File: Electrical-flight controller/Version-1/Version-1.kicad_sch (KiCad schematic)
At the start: 19 parts, among them J1 USB_B_Micro, U1 ESP32-WROOM-32, U2 W25Q32JVZP, U4 CP2102N-Axx-xQFN28, Y1 Crystal_GND24

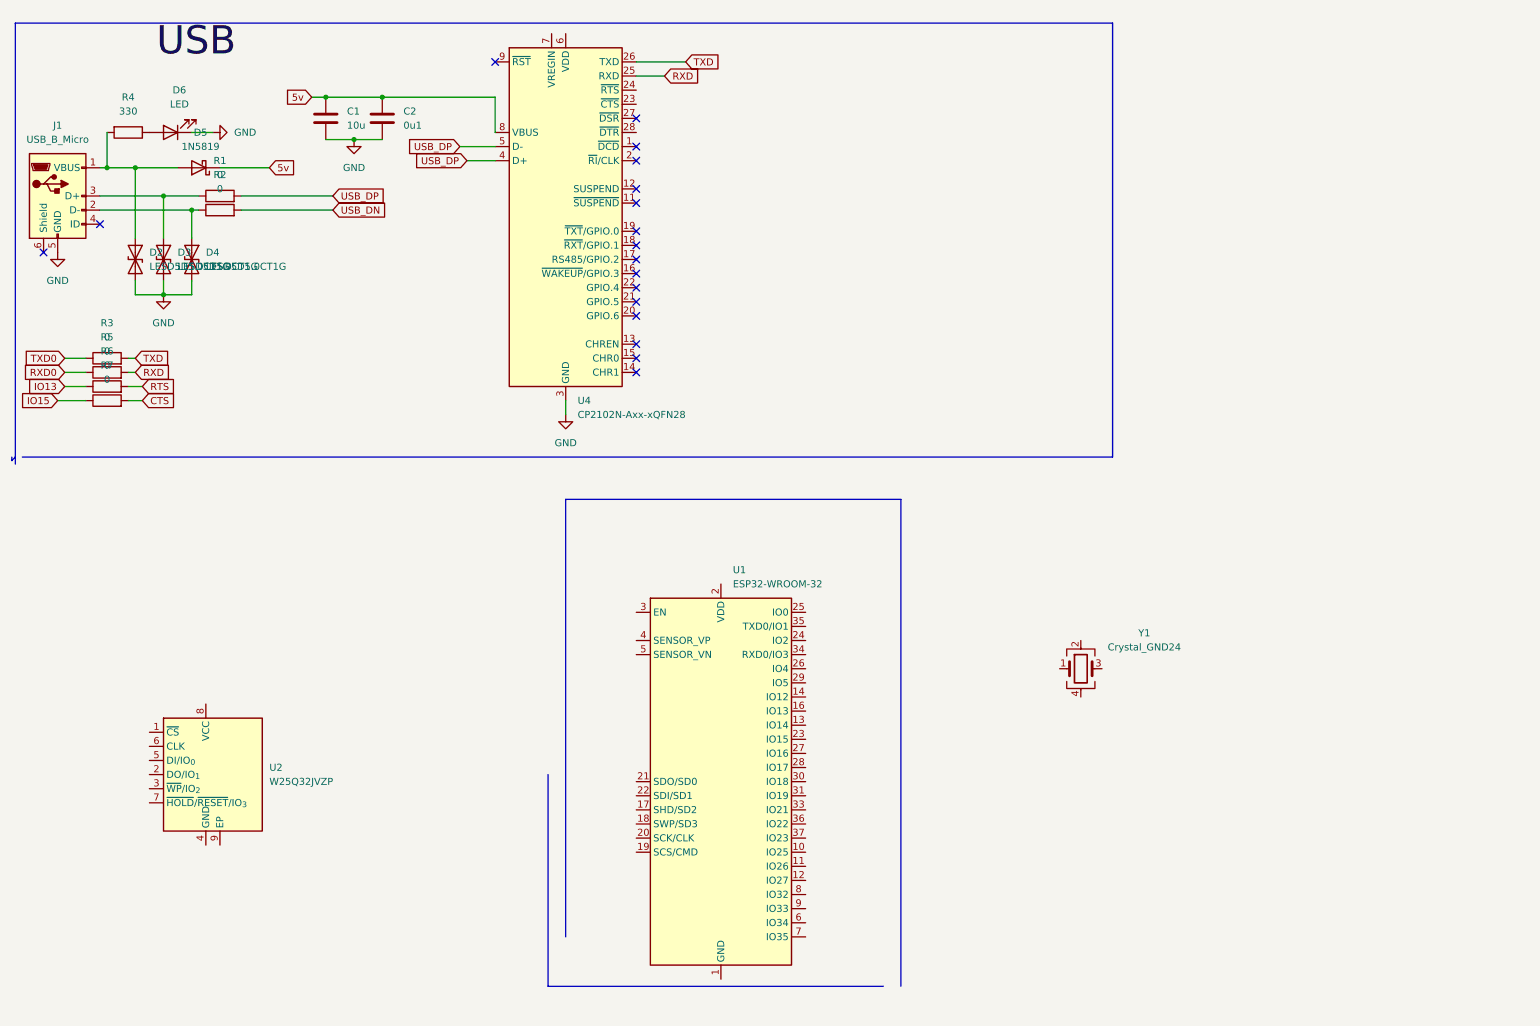
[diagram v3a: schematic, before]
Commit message: Pwoer supply
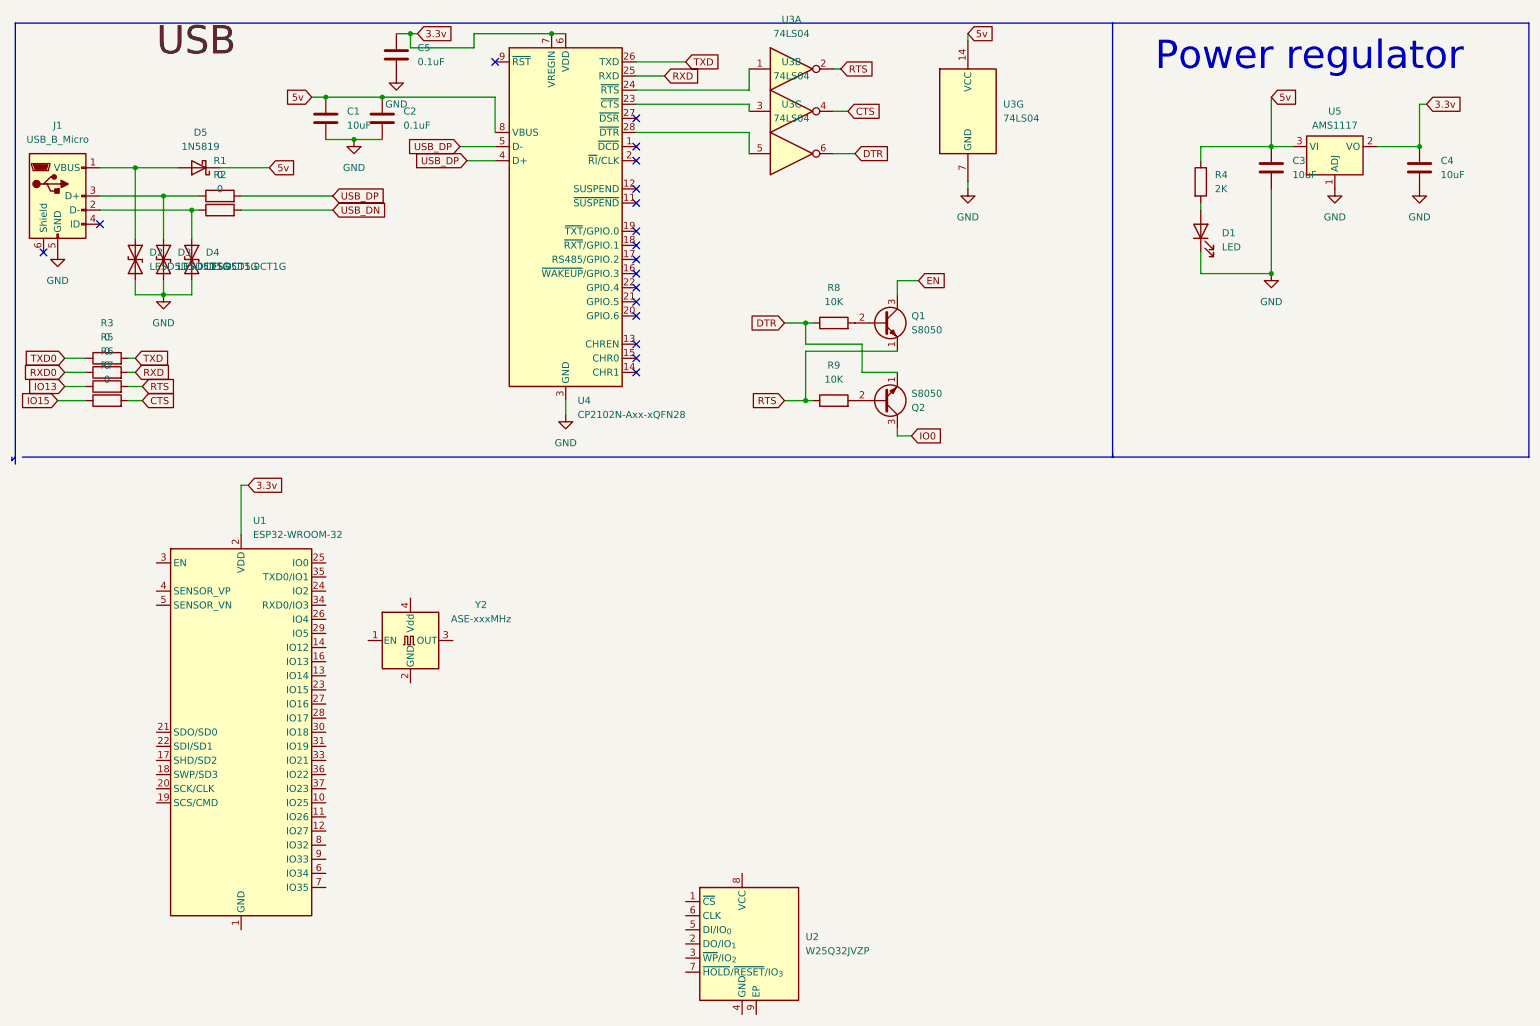
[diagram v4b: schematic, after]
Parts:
- removed D6: LED, LED_SMD:LED_0201_0603Metric, symbol Device:LED
- removed Y1: Crystal_GND24, symbol Device:Crystal_GND24
- added C3, C4: 10uF, symbol Device:C
- added C5: 0.1uF, symbol Device:C
- added D1: LED, symbol Device:LED
- added Q1, Q2: S8050, Package_TO_SOT_THT:TO-92_Inline, symbol Transistor_BJT:S8050
- added R8, R9: 10K, symbol Device:R
- added U3: 74LS04, symbol 74xx:74LS04
- added U5: AMS1117, Package_TO_SOT_SMD:SOT-223-3_TabPin2, symbol Regulator_Linear:AMS1117
- added Y2: ASE-xxxMHz, Oscillator:Oscillator_SMD_Abracon_ASE-4Pin_3.2x2.5mm, symbol Oscillator:ASE-xxxMHz
- C1: value 10u -> 10uF
- C2: value 0u1 -> 0.1uF
- R4: value 330 -> 2K; footprint Resistor_SMD:R_0402_1005Metric -> (none)
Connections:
- net 5v: now also R4.1, C3.1, U3.14 (VCC), U5.3 (VI)
- net CTS: now also U3.4
- net GND: now also C3.2, C4.2, C5.2, D1.1 (K), U3.7 (GND), U5.1 (ADJ)
- net RTS: now also Q1.1 (E), R9.1, U3.2
- net at D2.1 (A1), D5.2 (A), J1.1 (VBUS): no longer R4.2
- net at U4.23 (~{CTS}): now also U3.3
- net at U4.24 (~{RTS}): now also U3.1
- net at U4.28 (~{DTR}): now also U3.5
- net 3.3v: now reaches U4.6 (VDD)
- net 3.3v: now also U1.2 (VDD), U4.7 (VREGIN), C4.1, C5.1, U5.2 (VO)
- new net: Q2.2 (B), R9.2
- new net: D1.2 (A), R4.2
- new net: Q1.2 (B), R8.2
- new net DTR: Q2.1 (E), R8.1, U3.6
- new net EN: Q1.3 (C)
- new net IO0: Q2.3 (C)
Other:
- note added: "Power regulator"
- moved on the sheet: U1, U2

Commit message: flash chip, reset switches , mc etc
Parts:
- removed U2: W25Q32JVZP, Package_SON:WSON-8-1EP_6x5mm_P1.27mm_EP3.4x4.3mm, symbol Memory_Flash:W25Q32JVZP
- removed Y2: ASE-xxxMHz, Oscillator:Oscillator_SMD_Abracon_ASE-4Pin_3.2x2.5mm, symbol Oscillator:ASE-xxxMHz
- added BZ1: Buzzer, Buzzer_Beeper:MagneticBuzzer_Kingstate_KCG0601, symbol Device:Buzzer
- added C10, C11: 22p, Capacitor_SMD:C_0201_0603Metric, symbol Device:C
- added C6: 0.1uF, symbol Device:C
- added C7, C8: 1nF, symbol Device:C
- added C9: 0u1, Capacitor_SMD:C_0201_0603Metric, symbol Device:C
- added D6: ESD3.3V88D-C, symbol Device:D_TVS
- added J2, J3: Conn_01x02_Pin, symbol Connector:Conn_01x02_Pin
- added JP3, JP4: Jumper_2_Small_Open, Jumper:SolderJumper-2_P1.3mm_Open_Pad1.0x1.5mm, symbol Jumper:Jumper_2_Small_Open
- added Q4: BSS138, Package_TO_SOT_SMD:SOT-23, symbol Transistor_FET:BSS138
- added R10, R11, R12, R13: 100R, symbol Device:R
- added R14: 10K, symbol Device:R
- added R15, R16: 47R, symbol Device:R
- added R17, R18, R34: 2k2, Resistor_SMD:R_0402_1005Metric, symbol Device:R
- added R19, R20: 4k7, Resistor_SMD:R_0402_1005Metric, symbol Device:R
- added R21: 10k, Resistor_SMD:R_0402_1005Metric, symbol Device:R
- added SW1, SW2: SW_MEC_5G, symbol Switch:SW_MEC_5G
- added U2: W25Q128JVE, Package_SON:WSON-8-1EP_8x6mm_P1.27mm_EP3.4x4.3mm, symbol Memory_Flash:W25Q128JVE
- added U6: BMP390L, barometer:XDCR_BMP390L.kicad_mod, symbol BMP390L:BMP390L
- added U8: BNO055, Package_LGA:LGA-28_5.2x3.8mm_P0.5mm, symbol Sensor_Motion:BNO055
- added Y1: Crystal, Crystal:Crystal_C26-LF_D2.1mm_L6.5mm_Vertical, symbol Device:Crystal
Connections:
- net 3.3v: now also D6.1 (A1), R14.1, U2.8 (VCC)
- net EN: now also U1.3 (EN), C6.1, R14.2, R16.1
- net GND: now also U1.1 (GND), U1.15 (GND), U1.38 (GND), U1.39 (GND), C10.2, C11.2, C6.2, C7.1, C8.1, C9.2, D6.2 (A2), JP4.2 (B), Q4.2 (S), R34.2, SW1.1 (A), SW1.2 (A), SW2.1 (A), SW2.2 (A), U6.3 (VSS/GND), U6.8 (VSS/GND), U6.9 (VSS/GND), U8.2 (GND), U8.25 (GNDIO)
- net IO0: now also U1.25 (IO0), R15.1
- net RXD0: now also U1.34 (RXD0/IO3)
- net TXD0: now also U1.35 (TXD0/IO1)
- net at U1.13 (IO14): now also R10.1
- net at U1.14 (IO12): now also R11.1
- net at U1.16 (IO13): now also R12.1
- net at U1.23 (IO15): now also R13.1
- net BUZZER: now reaches U1.24 (IO2)
- net BUZZER: now also Q4.1 (G), R34.1
- new net: C10.1, U8.26 (XOUT32), Y1.2
- new net: C9.1, U8.9 (CAP)
- new net: J2.1 (Pin_1), R11.2
- new net: J2.2 (Pin_2), R10.2
- new net: BZ1.2 (-), Q4.3 (D)
- new net: J3.1 (Pin_1), R13.2
- new net: R21.1, U8.11 (~{RESET})
- new net: J3.2 (Pin_2), R12.2
- new net: C8.2, R16.2, SW2.3 (B), SW2.4 (B)
- new net: C11.1, U8.27 (XIN32), Y1.1
- new net: C7.2, R15.2, SW1.3 (B), SW1.4 (B)
- new net: JP3.1 (A), JP4.1 (A), U6.5 (SDO/DNC/SA0)
- new net +3.3V: BZ1.1 (+), JP3.2 (B), R17.1, R18.1, R19.1, R20.1, R21.2, U6.1 (VDDIO), U6.10 (VDD), U6.6 (~{CS}), U8.28 (VDDIO), U8.3 (VDD)
- new net SCL: R18.2, R20.2, U6.2 (SCK/SCL), U8.17 (COM3)
- new net SDA: R17.2, R19.2, U6.4 (SDI/SDO/SDA), U8.18 (COM2)
- no-connect marks 18 -> 26

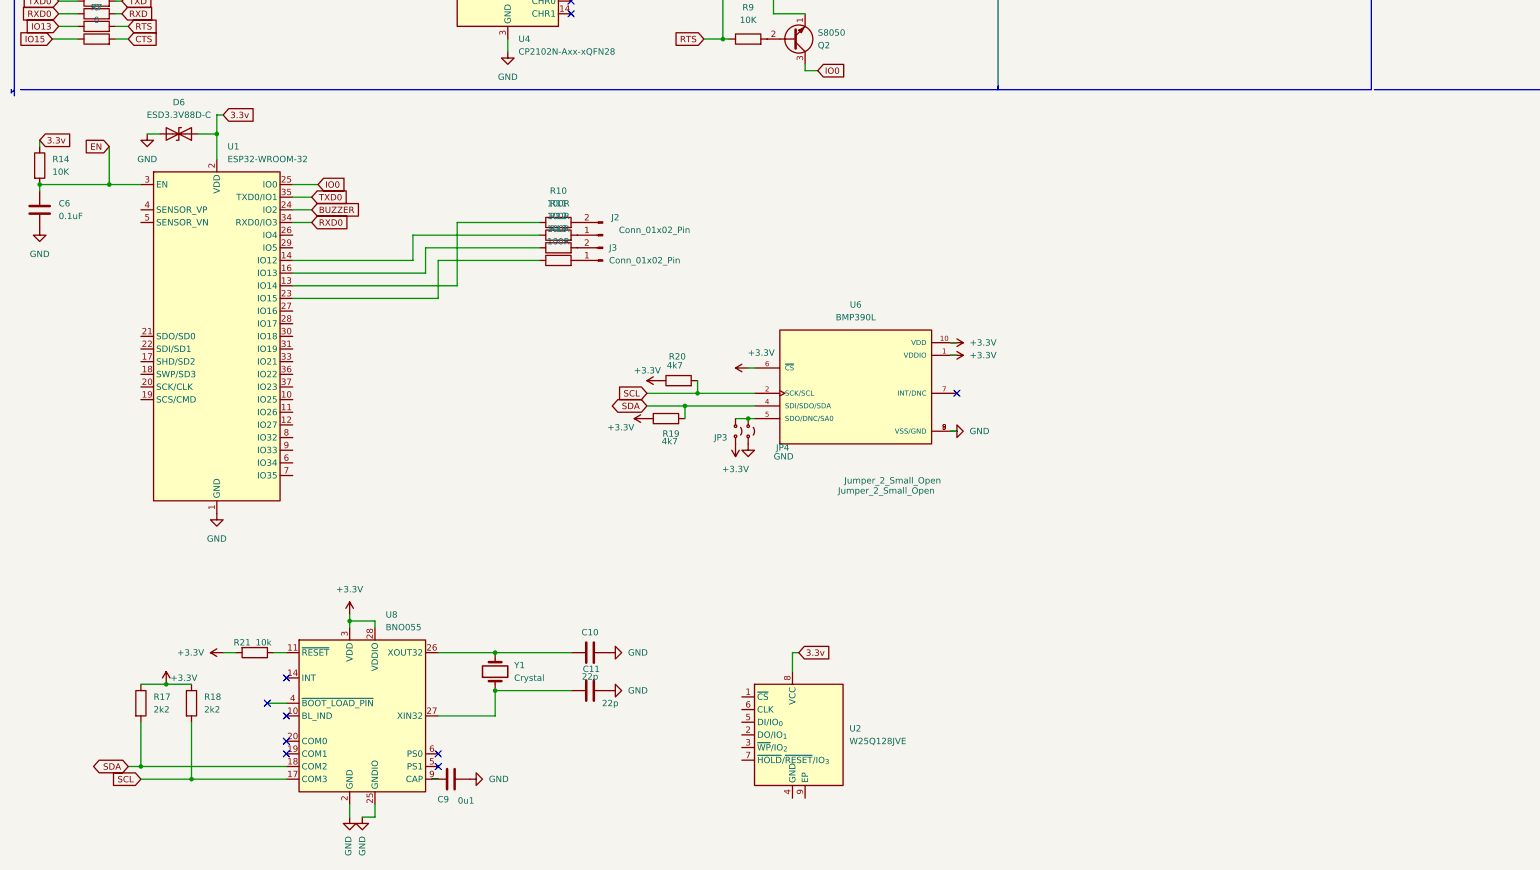
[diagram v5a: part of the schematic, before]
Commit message: 123
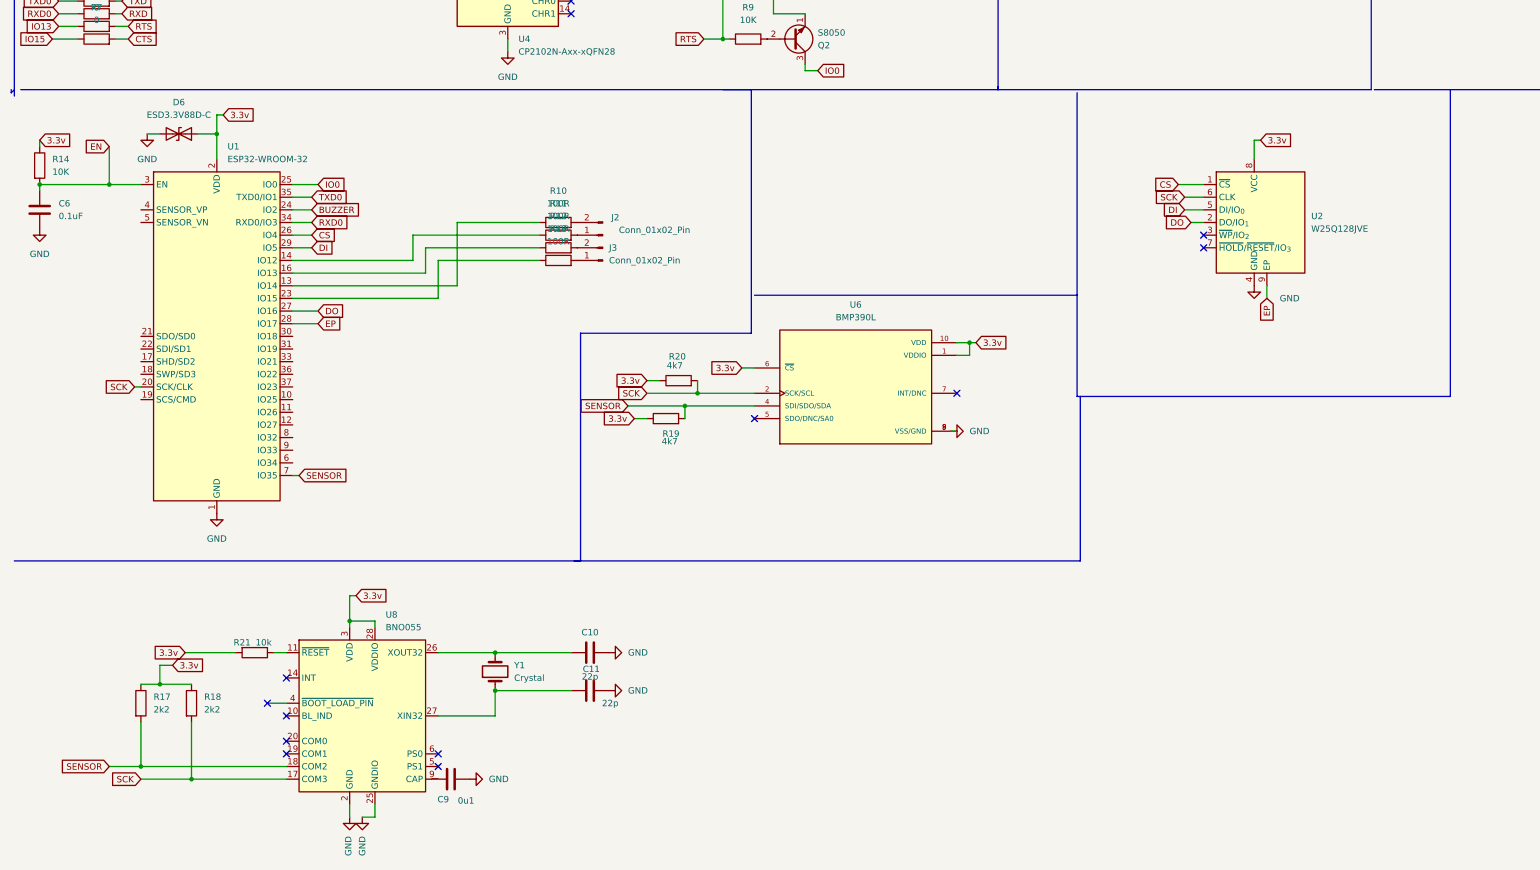
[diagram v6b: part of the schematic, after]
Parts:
- removed JP3, JP4: Jumper_2_Small_Open, Jumper:SolderJumper-2_P1.3mm_Open_Pad1.0x1.5mm, symbol Jumper:Jumper_2_Small_Open
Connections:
- net SCL is gone; now on net SCK: R18.2, R20.2, U6.2 (SCK/SCL), U8.17 (COM3)
- net SDA is gone; now on net SENSOR: R17.2, R19.2, U6.4 (SDI/SDO/SDA), U8.18 (COM2)
- net +3.3V: no longer R17.1, R18.1, R19.1, R20.1, R21.2, U6.1 (VDDIO), U6.10 (VDD), U6.6 (~{CS}), U8.28 (VDDIO), U8.3 (VDD)
- net 3.3v: now also R17.1, R18.1, R19.1, R20.1, R21.2, U6.1 (VDDIO), U6.10 (VDD), U6.6 (~{CS}), U8.28 (VDDIO), U8.3 (VDD)
- net GND: now also U2.4 (GND)
- net CS: now reaches U2.1 (~{CS})
- net CS: now also U1.26 (IO4)
- net DO: now reaches U2.2 (DO/IO_{1})
- net DO: now also U1.27 (IO16)
- net DI: now reaches U2.5 (DI/IO_{0})
- net DI: now also U1.29 (IO5)
- net SCK: now reaches U2.6 (CLK)
- net SCK: now also U1.20 (SCK/CLK)
- net EP: now reaches U2.9 (EP)
- net EP: now also U1.28 (IO17)
- net SENSOR: now reaches U1.7 (IO35)
- no-connect marks 26 -> 29
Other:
- moved on the sheet: U2
